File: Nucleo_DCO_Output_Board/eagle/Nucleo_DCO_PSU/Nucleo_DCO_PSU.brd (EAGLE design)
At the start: 94 x 71.1 mm, 38 parts, among them CN1 9VPWR, IC1 TLE2426LP, IC2 NJM4580, IC3 NJM4580

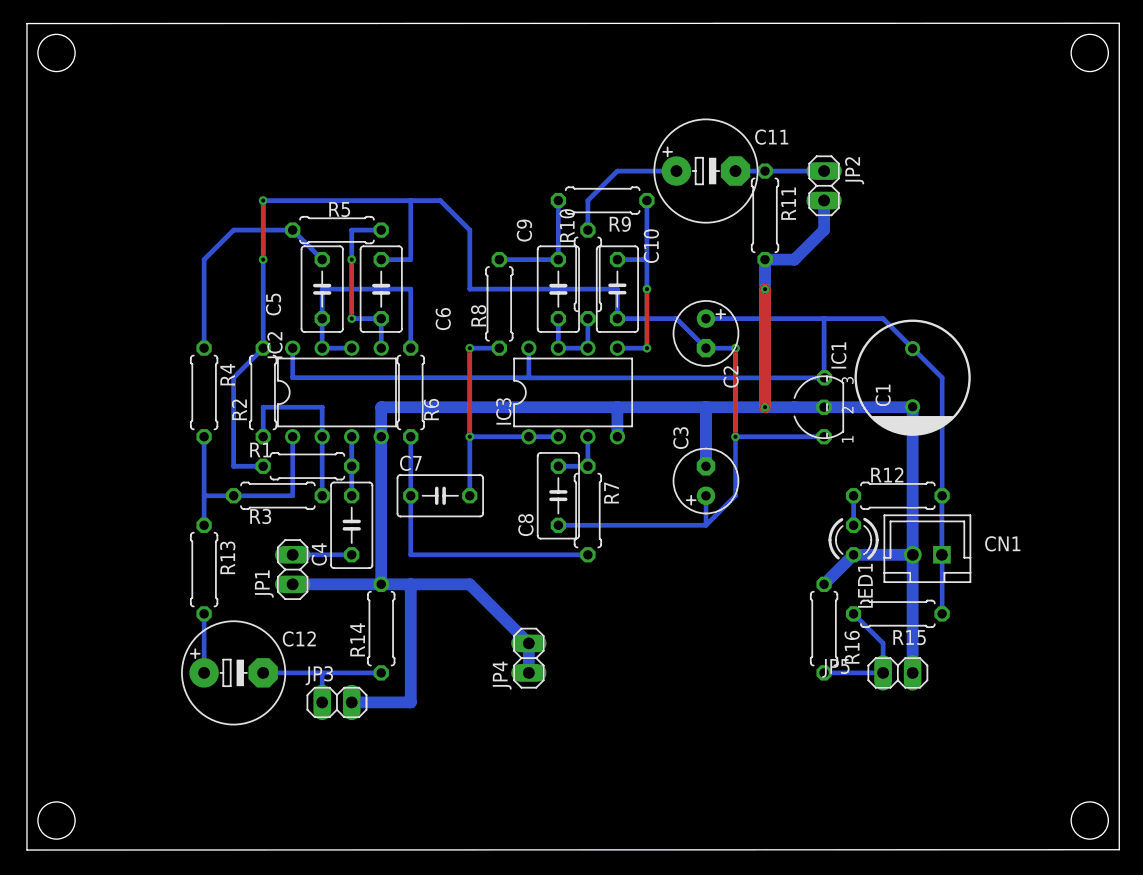
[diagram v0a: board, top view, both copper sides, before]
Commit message: Nucleo_DCO_PSU
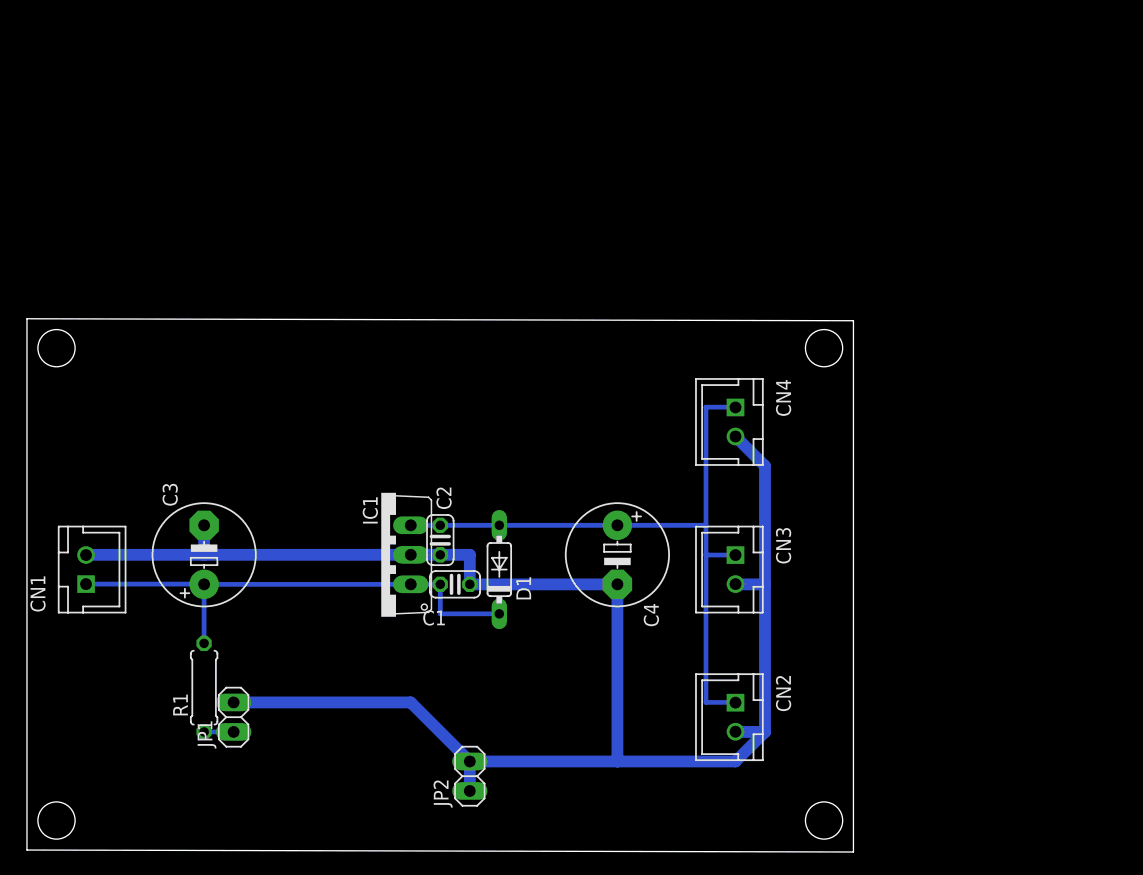
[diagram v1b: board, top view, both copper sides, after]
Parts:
- removed C10: 220pF, rcl:C050-035X075
- removed C11, C12: 100uF, rcl:E5-8,5
- removed C5, C7, C9: 0.001uF, rcl:C050-035X075
- removed C6: 680pF, rcl:C050-035X075
- removed C8: 470pF, rcl:C050-035X075
- removed IC2, IC3: NJM4580, linear:DIL08
- removed JP3: BYPASS, pinhead:1X02
- removed JP4: TP_GND, pinhead:1X02
- removed JP5: PW_WATCH, pinhead:1X02
- removed LED1: (no value), led:LED3MM
- removed R10, R13: 100, rcl:0207/7
- removed R11, R14: 100k, rcl:0207/7
- removed R12, R2: 10k, rcl:0207/7
- removed R15: 120k, rcl:0207/7
- removed R16: 33k, rcl:0207/7
- removed R3: 20k, rcl:0207/7
- removed R4, R6, R8: 12k, rcl:0207/7
- removed R5: 3.3k, rcl:0207/7
- removed R7: 3.9k, rcl:0207/7
- removed R9: 6.8k, rcl:0207/7
- added CN2, CN3, CN4: PWR_OUT, jst-xh:B2B-XH-A
- added D1: 1S4, diode:DO35-7
- C1: value 470uF -> 0.33uF; device rcl:SANYO-OSCON_F13 -> rcl:C025-024X044
- C2: value 10uF -> 0.1uF; device rcl:E2,5-6 -> rcl:C025-024X044
- C3: value 10uF -> 100uF; device rcl:E2,5-6 -> rcl:E5-8,5
- C4: value 1uF -> 100uF; device rcl:C050-035X075 -> rcl:E5-8,5
- CN1: value 9VPWR -> PWR_IN
- IC1: value TLE2426LP -> 7809TV; device mylib2:TO226AA -> linear:TO220V
- JP1: value IN -> LED
- JP2: value OUT -> TP_GND
- R1: value 100k -> 1k
- moved CN1 72.4 mm to (5.08, 24.1), turned to 90 degrees
- moved JP2 59.2 mm to (38.1, 6.35), turned to 90 degrees
- moved C3 43.6 mm to (15.2, 25.4)
- moved C1 43.2 mm to (36.8, 22.9), turned to 0 degrees
- moved IC1 40.2 mm to (30.5, 25.4)
- moved C2 29.0 mm to (35.6, 26.7)
- moved C4 23.0 mm to (50.8, 25.4), turned to 270 degrees
- moved R1 21.0 mm to (15.2, 14.0), turned to 90 degrees
- moved JP1 13.7 mm to (17.8, 11.4), turned to 90 degrees
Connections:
- removed net N$10: C8.2, IC3.3, R7.1
- removed net N$11: C7.1, R6.1, R7.2
- removed net N$12: LED1.A, R12.2
- removed net N$13: C7.2, IC3.1, IC3.2, R8.2
- removed net N$14: C10.2, IC3.5, R9.1
- removed net N$15: C9.1, R8.1, R9.2
- removed net N$16: C9.2, IC3.6, IC3.7, R10.2
- removed net N$18: C12.+, R13.2
- removed net N$19: C12.-, JP3.1, R14.1
- removed net N$2: IC2.2, R2.1, R3.2
- removed net N$20: JP5.1, R15.2, R16.1
- removed net N$5: C4.2, IC2.3, R1.2
- removed net N$6: C5.1, R4.1, R5.2
- removed net N$7: C11.+, R10.1
- removed net N$8: C11.-, JP2.1, R11.1
- removed net N$9: C5.2, IC2.6, IC2.7, R6.2
- removed net VCC: C1.+, C2.+, CN1.1, IC1.3, IC2.8, IC3.8, R12.1, R15.1
- removed net VCC/2: C10.1, C2.-, C3.+, C6.1, C8.1, IC1.1, R1.1, R2.2
- net GND: now also C1.2, C2.2, C4.-, CN2.2, CN3.2, CN4.2, JP2.1; no longer C1.-, IC2.4, IC3.4, JP3.2, JP4.1, JP4.2, JP5.2, LED1.K, R11.2, R14.2, R16.2
- net N$1: now also JP1.1, R1.1; no longer IC2.1, R13.1, R3.1, R4.2
- net N$3: now also C1.1, C3.+, CN1.1, D1.C, IC1.1, R1.2; no longer C6.2, IC2.5, R5.1
- net N$4: now also C2.1, C4.+, CN2.1, CN3.1, CN4.1, D1.A, IC1.3; no longer C4.1, JP1.1
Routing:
- net VCC/2: track 123.6 -> 0.00 mm, vias 4 -> 0
- net VCC: track 98.8 -> 0.00 mm
- net N$4: track 5.08 -> 58.5 mm
- net N$3: track 15.2 -> 43.2 mm, vias 2 -> 0
- net N$11: track 25.4 -> 0.00 mm
- net N$13: track 22.9 -> 0.00 mm, vias 2 -> 0
- net N$9: track 20.3 -> 0.00 mm
- net N$6: track 19.9 -> 0.00 mm
- net N$14: track 17.8 -> 0.00 mm, vias 2 -> 0
- net N$1: track 20.3 -> 2.54 mm
- net N$2: track 15.2 -> 0.00 mm
- net GND: track 161.8 -> 149.0 mm, vias 2 -> 0
- net N$19: track 12.7 -> 0.00 mm
- net N$7: track 11.2 -> 0.00 mm
- net N$20: track 11.2 -> 0.00 mm
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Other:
- board size 94 x 71.1 mm -> 71.1 x 45.9 mm
- board text added: "Nucleo DCO PSU"
- board text removed: "Nucleo DCO Output Board"
